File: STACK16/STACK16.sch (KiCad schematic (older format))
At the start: 43 parts, among them J1 Conn_01x09_Male, J2 Conn_01x09_Male, J3 Conn_01x01_Male, J4 Conn_01x01_Male, J5 Conn_01x09_Male, J6 Conn_01x09_Male, U1 74LS574, U2 74LS574

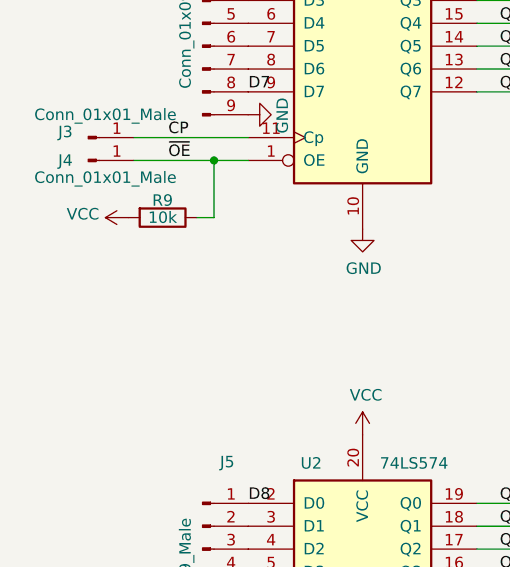
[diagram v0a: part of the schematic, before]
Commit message: Polishing Stack16
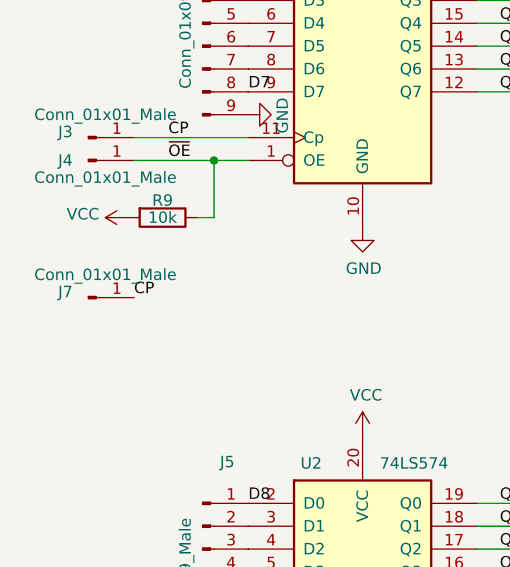
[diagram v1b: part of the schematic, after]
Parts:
- added J7: Conn_01x01_Male, Connector_PinHeader_2.54mm:PinHeader_1x01_P2.54mm_Horizontal, symbol Connector:Conn_01x01_Male
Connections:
- net CP: now also J7.1 (Pin_1)
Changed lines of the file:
@@
 Wire Wire Line
 	1500 5400 2000 5400
+$Comp
+L Connector:Conn_01x01_Male J7
+U 1 1 6653500A
+P 1300 3500
+F 0 "J7" H 1200 3525 50  0000 C CNN
+F 1 "Conn_01x01_Male" H 1375 3600 50  0000 C CNN
+F 2 "Connector_PinHeader_2.54mm:PinHeader_1x01_P2.54mm_Horizontal" H 1300 3500 50  0001 C CNN
+F 3 "~" H 1300 3500 50  0001 C CNN
+	1    1300 3500
+	1    0    0    -1
+$EndComp
+Text Label 1500 3500 0    50   ~ 0
+CP
 $EndSCHEMATC

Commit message: Polishing STACK16
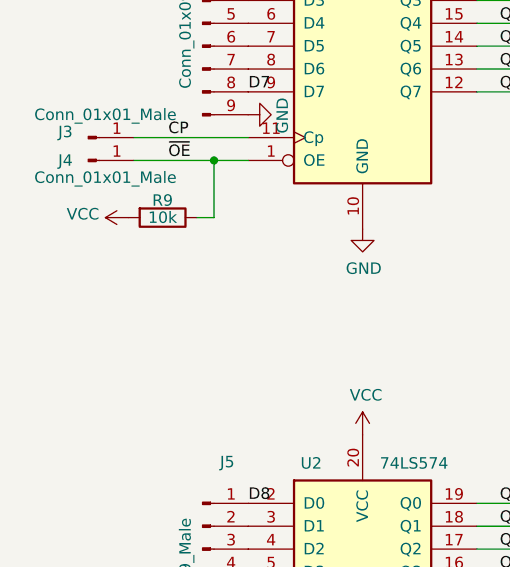
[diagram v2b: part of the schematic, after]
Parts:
- removed J7: Conn_01x01_Male, Connector_PinHeader_2.54mm:PinHeader_1x01_P2.54mm_Horizontal, symbol Connector:Conn_01x01_Male
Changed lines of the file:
@@
 Wire Wire Line
 	1500 5400 2000 5400
-$Comp
-L Connector:Conn_01x01_Male J7
-U 1 1 6653500A
-P 1300 3500
-F 0 "J7" H 1200 3525 50  0000 C CNN
-F 1 "Conn_01x01_Male" H 1375 3600 50  0000 C CNN
-F 2 "Connector_PinHeader_2.54mm:PinHeader_1x01_P2.54mm_Horizontal" H 1300 3500 50  0001 C CNN
-F 3 "~" H 1300 3500 50  0001 C CNN
-	1    1300 3500
-	1    0    0    -1
-$EndComp
-Text Label 1500 3500 0    50   ~ 0
-CP
 $EndSCHEMATC
